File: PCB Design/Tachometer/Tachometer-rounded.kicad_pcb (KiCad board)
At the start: 2 copper layers, 38.1 x 32.2 mm, 52 parts, among them J1 OLED Display Socket, J2 Boot0, J3 USB_B_Micro, J4 UART, J5 SWD, J6 PB_12, J7 PB_13, J8 PB_14, J9 PB_15, SW1 POWER, SW2 Reset, SW3 Mode_1, SW4 Mode_2, U1 AMS1117-3.3, U2 LMV321, U3 STM32F103C8Tx, Y1 8MHz_Crystal

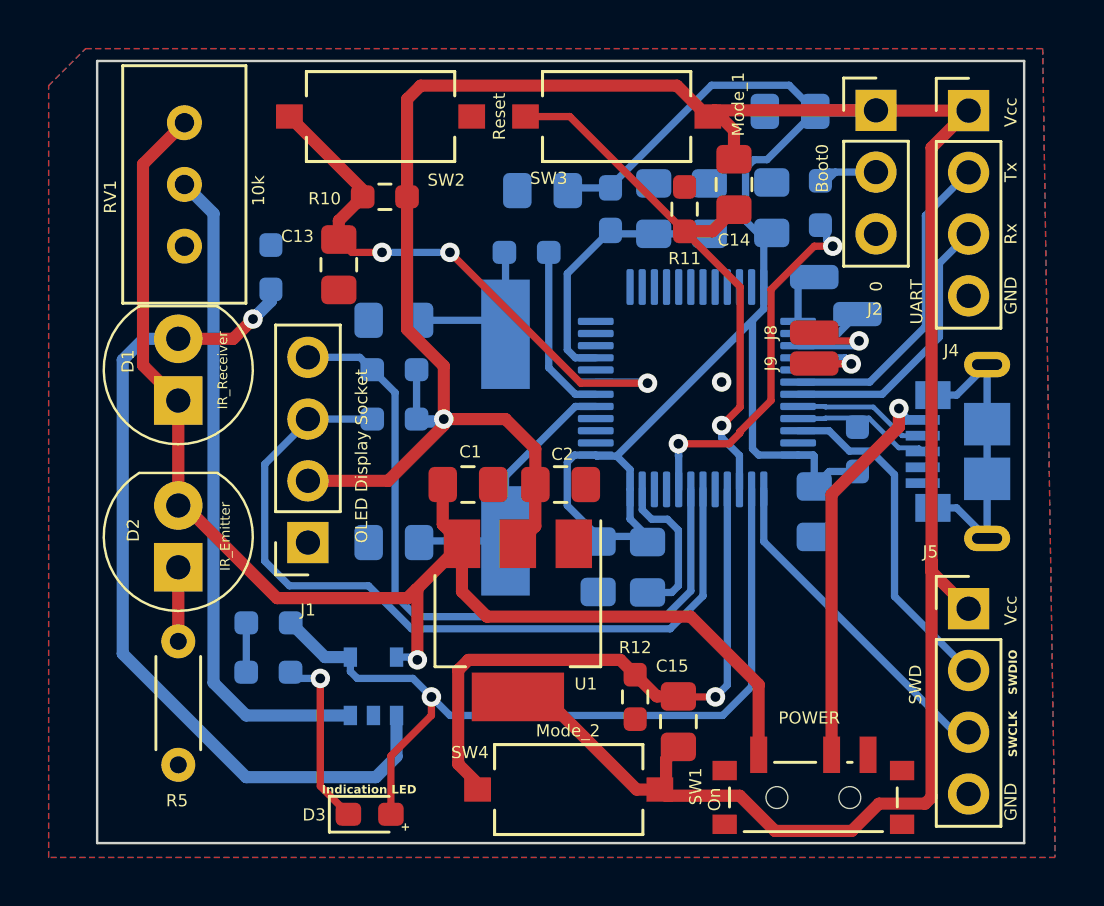
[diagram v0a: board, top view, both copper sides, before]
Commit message: Routed
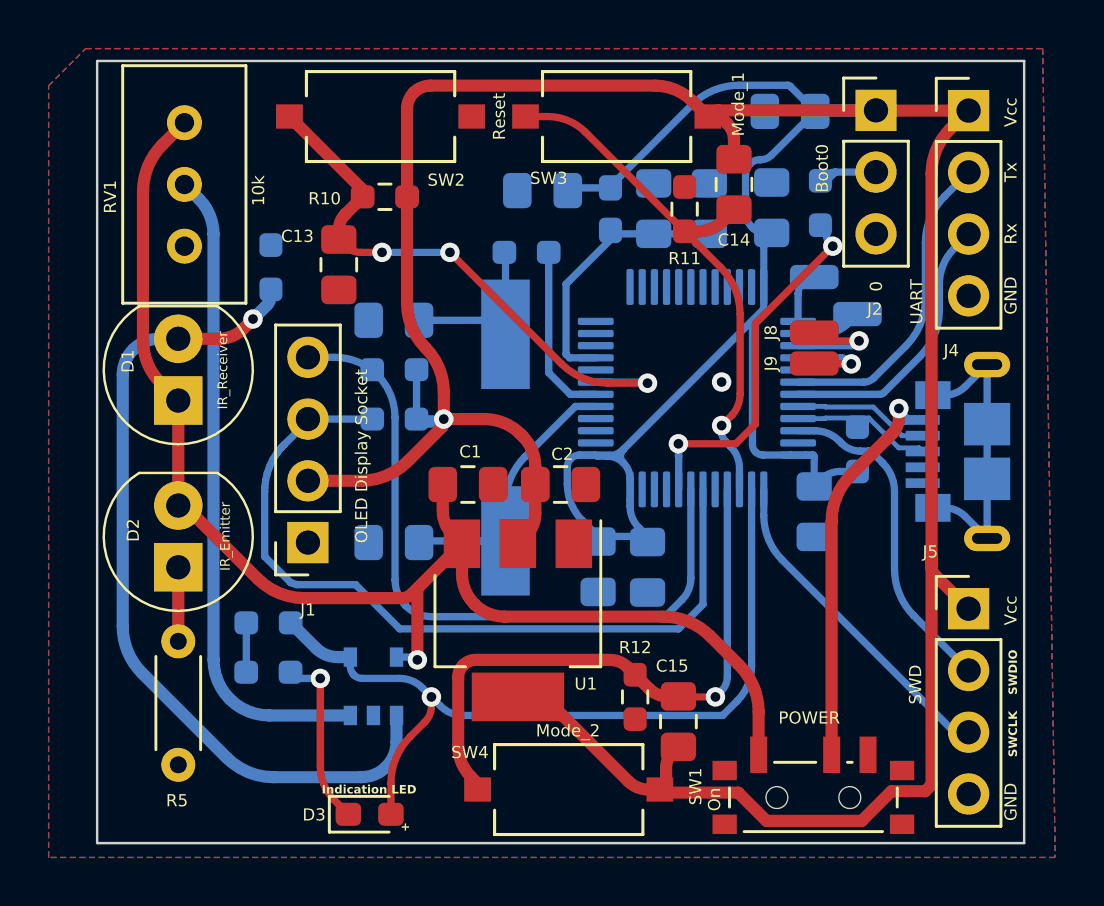
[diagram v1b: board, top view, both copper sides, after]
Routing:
- net GND: track 8.38 -> 2.03 mm
- net /VDD: track 169.5 -> 166.9 mm
- net /VCC: track 57.0 -> 55.4 mm
- net /OP_Out: track 35.0 -> 34.4 mm
- net Net-(D1-A): track 35.1 -> 34.4 mm
- net /HSE_IN: track 11.1 -> 10.5 mm
- net Net-(C12-Pad1): track 7.29 -> 6.78 mm
